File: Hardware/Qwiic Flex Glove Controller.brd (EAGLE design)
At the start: 25.4 x 36.8 mm, 43 parts, among them U1 ADS1015, U4 LMV358

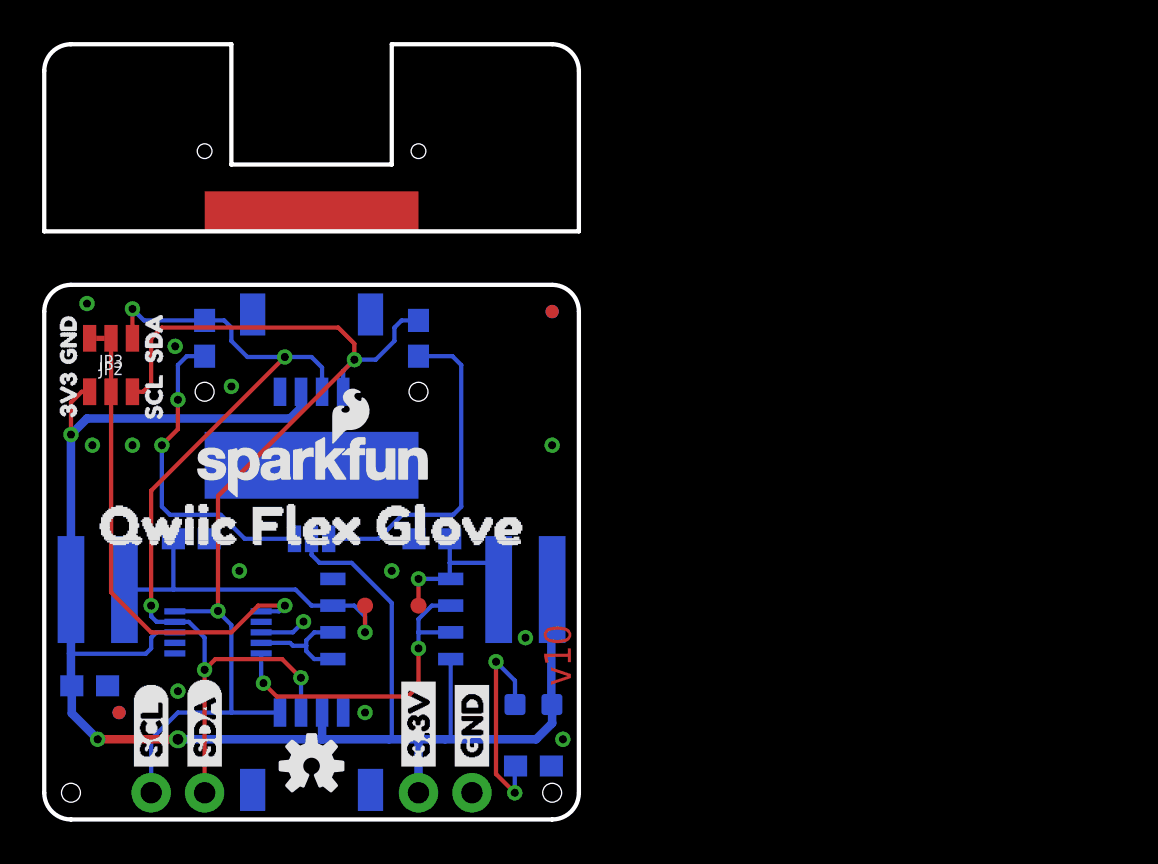
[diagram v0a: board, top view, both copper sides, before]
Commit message: cleaned repo
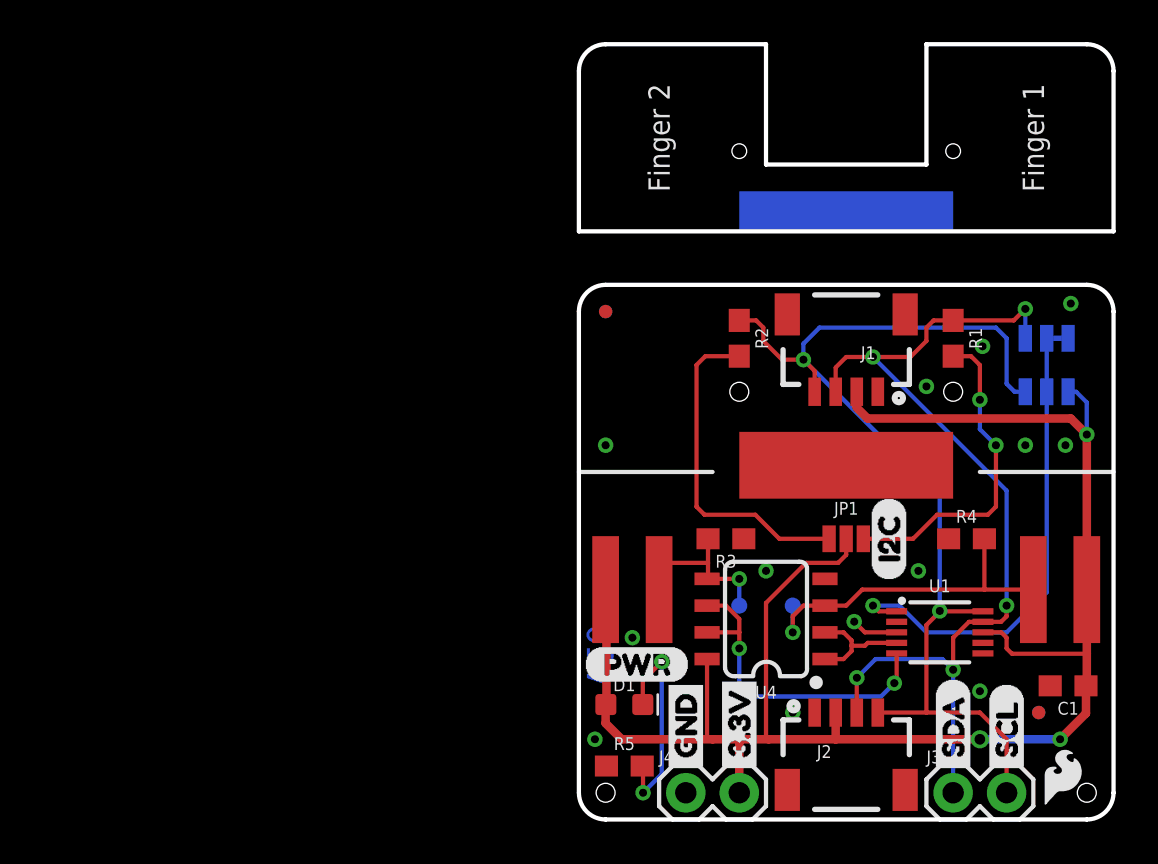
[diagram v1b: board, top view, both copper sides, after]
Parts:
- moved U$14 48.8 mm to (24.4, 14.0), flipped to the bottom
- moved U$3 48.5 mm to (24.3, 18.4), flipped to the bottom
- moved U$4 48.5 mm to (24.3, 21.0), flipped to the bottom
- moved C1 46.5 mm to (23.2, 6.35), flipped to the top
- moved R6 45.7 mm to (22.9, 12.2), flipped to the top
- moved JP2 44.5 mm to (22.2, 22.9), flipped to the bottom
- moved JP3 44.5 mm to (22.2, 20.3), flipped to the bottom
- moved FD1 43.7 mm to (21.8, 5.08), flipped to the top
- moved FD2 43.7 mm to (21.8, 5.08), flipped to the bottom
- moved LOGO3 43.7 mm to (21.8, 0.38), flipped to the top
- moved U$10 40.6 mm to (20.3, 2.03), flipped to the bottom
- moved U$9 40.6 mm to (20.3, 2.03), flipped to the top
- moved U$12 40.4 mm to (20.2, 21.0), flipped to the bottom
- moved U$13 40.4 mm to (20.2, 18.3), flipped to the bottom
- moved LOGO1 37.1 mm to (18.5, 15.2), flipped to the bottom
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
